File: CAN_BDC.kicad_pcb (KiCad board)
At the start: 2 copper layers, 26 x 28.5 mm, 35 parts, among them P1 CONN_01X02, P2 CONN_01X05, P3 CONN_01X02, P4 CONN_01X02, P5 CONN_01X02, P6 CONN_01X02, P7 CONN_01X04, P8 CONN_01X01, P9 CONN_01X02, U1 PSD2CAN, U2 SN65HVD232D, U3 POLOLU_A4988, U4 STM32F042G4U6, U5 MC33063

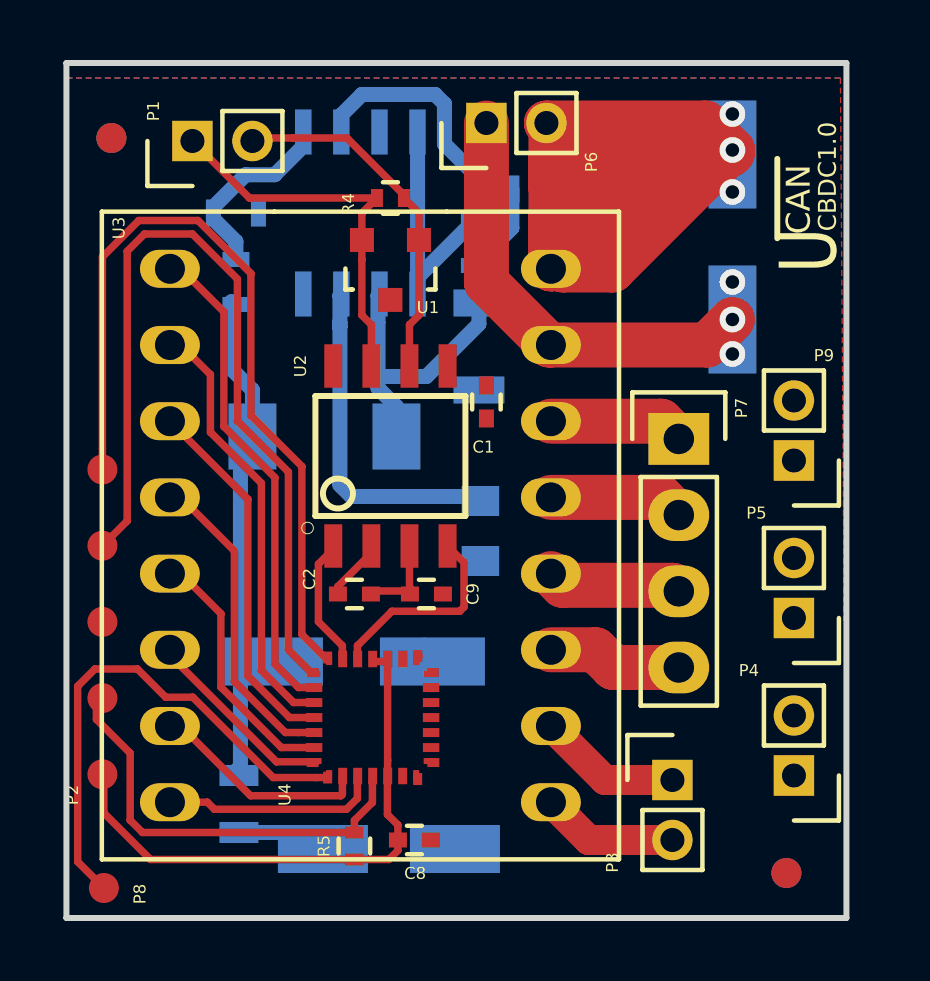
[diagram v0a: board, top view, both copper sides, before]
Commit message: Root full
Root full
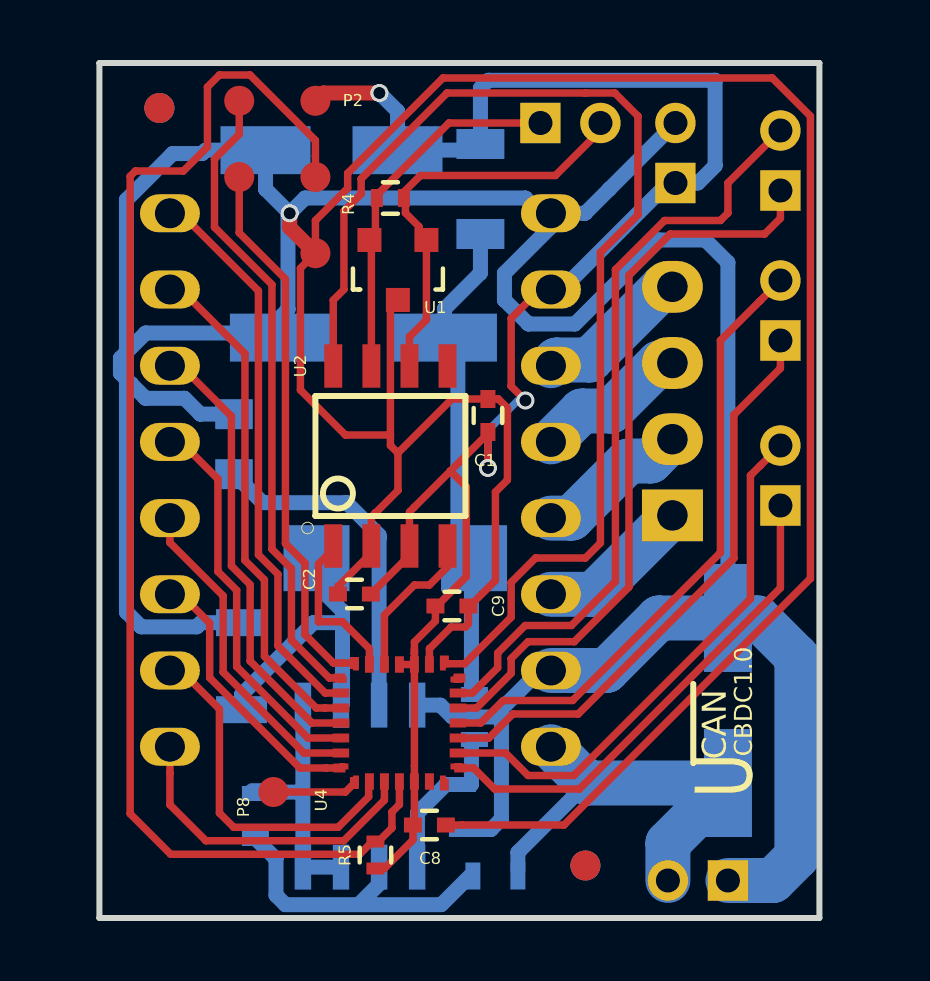
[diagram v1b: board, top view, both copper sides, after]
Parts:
- L1: footprint usb_ccb_custom:DE0704_Coil -> usb_ccb_custom:DE0704_Coil_2
- L2: footprint Resistors_SMD:R_0805 -> Capacitors_SMD:C_1206
- P1, P3, P4, P5, P6, P7, P9, U3: moved to B.Cu
- P2: footprint usb_ccb_custom:swd_smd_conn5 -> usb_ccb_custom:swd_smd_conn5_x2
- moved P6 26.5 mm to (159.4, 110.3)
- moved C7 23.4 mm to (146.2, 86.0), turned to 180 degrees
- moved R6 22.9 mm to (151.7, 110.2)
- moved L2 22.0 mm to (151.2, 87.2), turned to 90 degrees
- moved R1 21.2 mm to (150.6, 107.8), turned to 270 degrees
- moved R2 20.4 mm to (143.7, 108.2)
- moved P2 19.9 mm to (145.7, 84.3), turned to 270 degrees
- moved P3 19.9 mm to (157.7, 87.0)
- moved U5 19.1 mm to (147.2, 107.2), turned to 0 degrees
- moved R3 16.5 mm to (151.0, 104.8), turned to 90 degrees
- moved C4 15.5 mm to (159.4, 104.3), turned to 270 degrees
- moved D1 13.3 mm to (143.2, 103.2), turned to 90 degrees
- moved P1 11.6 mm to (153.2, 85.0), turned to 270 degrees
- moved C6 10.8 mm to (147.3, 92.2), turned to 180 degrees
- moved P5 9.26 mm to (161.2, 92.3), turned to 0 degrees
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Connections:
- U4 pad 2: DRV_STEP -> DRV_MS1
- U4 pad 23: DRV_nENABLE -> DRV_DIR
- U4 pad 24: DRV_MS1 -> DRV_STEP
- U4 pad 25: DRV_MS2 -> DRV_nSLEEP
- U4 pad 26: DRV_MS3 -> DRV_nRESET
- U4 pad 27: DRV_nRESET -> DRV_MS3
- U4 pad 28: DRV_nSLEEP -> DRV_MS2
- U4 pad 3: DRV_DIR -> DRV_nENABLE
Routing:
- net GND: track 23.7 -> 196.3 mm, vias 3 -> 1
- net CAN_MOD: track 0.57 -> 40.1 mm
- net VPP: track 47.8 -> 14.3 mm, vias 3 -> 0
- net Net-(P2-Pad2): track 14.2 -> 43.4 mm
- net +3V3: track 30.7 -> 58.2 mm, vias 0 -> 3
- net /GPIO4: track 0.00 -> 25.5 mm
- net /GPIO3: track 0.00 -> 24.8 mm
- net /GPIO2: track 0.00 -> 21.0 mm
- net /GPIO1: track 0.00 -> 19.6 mm
- net /USART_RX: track 0.00 -> 18.0 mm
- net /USART_TX: track 0.04 -> 16.5 mm
- net Net-(P8-Pad1): track 17.2 -> 2.82 mm
- net DRV_DIR: track 7.16 -> 18.9 mm
- net DRV_STEP: track 7.26 -> 17.0 mm
- net SW_DIO: track 27.2 -> 18.2 mm
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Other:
- board size 26 x 28.5 mm -> 24 x 28.5 mm
